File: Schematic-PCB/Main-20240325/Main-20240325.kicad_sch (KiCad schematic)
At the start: 104 parts, among them J1 Conn_01x10_Pin, J2 Conn_01x03_Pin, J3 Conn_01x15_Pin, J4 Conn_02x05_Odd_Even, U1 DEV-16771, U10 TSSP58038, U11 TSSP58038, U12 TSSP58038, U13 TSSP58038, U14 TSSP58038, U15 TSSP58038, U16 TSSP58038, U17 TSSP58038, U18 TSSP58038, U19 TSSP58038, U4 TSSP58038, U5 TSSP58038, U6 TSSP58038, U7 TSSP58038, U8 TSSP58038, U9 TSSP58038

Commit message: 回路/基板をいろいろ直した
具体的にはあんまり進んでないけど
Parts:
- removed JP2, JP4: Jumper_2_Small_Open, Jumper:SolderJumper-2_P1.3mm_Open_Pad1.0x1.5mm, symbol Jumper:Jumper_2_Small_Open
- added D19: D_Small, symbol Device:D_Small
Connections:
- net SW-TAC-5 is gone; now on net KickerSignal: J1.7 (Pin_7), U1.32 (OUT1B)
- net +5V: now also D19.2 (A); no longer U2.14 (5V)
- net SW-TAC-3: now also U1.31 (CTX3); no longer U1.35 (TX8)
- net SW-TAC-4: now also U1.30 (CRX3); no longer U1.34 (RX8)
- net at R5.2: now also U2.9 (SCK_D8); no longer U2.8 (RX_D7)
- net Main-RX2: now reaches U2.7 (TX_D6)
- net Main-RX2: now also U1.7 (RX2)
- net Cam-main=RX renamed Cam-TX
- net Cam-TX: now also U1.34 (RX8); no longer U1.7 (RX2)
- net Cam-main=TX renamed Cam-RX
- net Cam-RX: now also U1.35 (TX8); no longer U1.8 (TX2)
- net Cam_MISO_RX renamed Cam-MISO_RX
- net Cam_MOSI_TX renamed Cam-MOSI_TX
- net KickerSignal-main renamed KickerSignal
- net KickerSignal: no longer U1.30 (CRX3)
- net Line-MD-Main=RX_3.3V renamed Line-TX
- net Line-MD-Main=TX_3.3V renamed Line-RX
- new net: D19.1 (K), U2.14 (5V)
- new net Main-TX2: U1.8 (TX2), U2.8 (RX_D7)
- no-connect marks 27 -> 26
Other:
- note added: "UART"
- moved on the sheet: C1, C10, C11, C12, C13, C14, C15, C16, C17, C18, C19, C2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

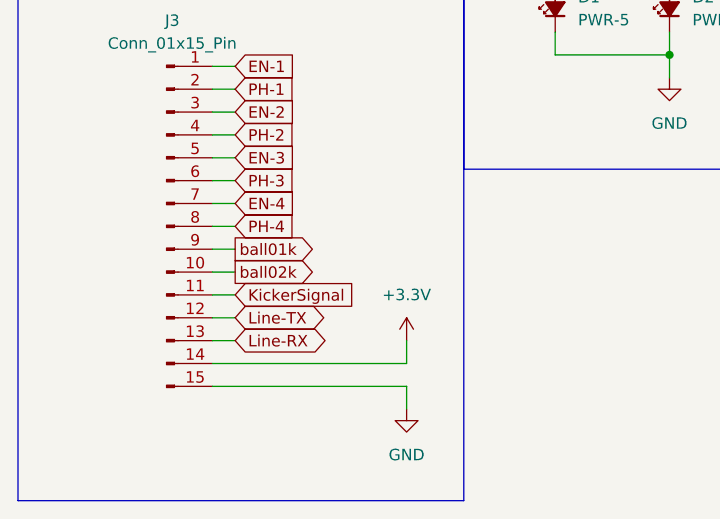
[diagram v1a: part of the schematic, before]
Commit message: MDのDRしたよ
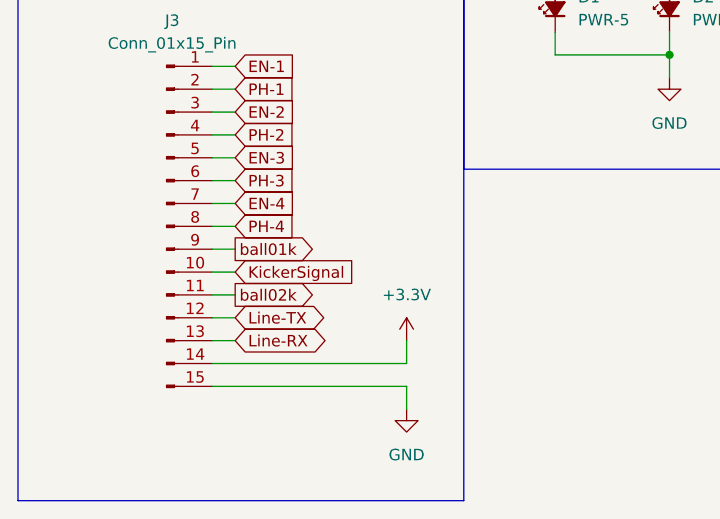
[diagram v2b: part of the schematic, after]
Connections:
- net KickerSignal: now also J3.10 (Pin_10); no longer J3.11 (Pin_11)
- net ball02k: now also J3.11 (Pin_11); no longer J3.10 (Pin_10)
